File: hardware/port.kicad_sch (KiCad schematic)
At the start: 13 parts, among them J1 USB_A_Stacked, Q1 AO3401A, Q2 AO3401A, Q3 MMBT3904, Q4 MMBT3904

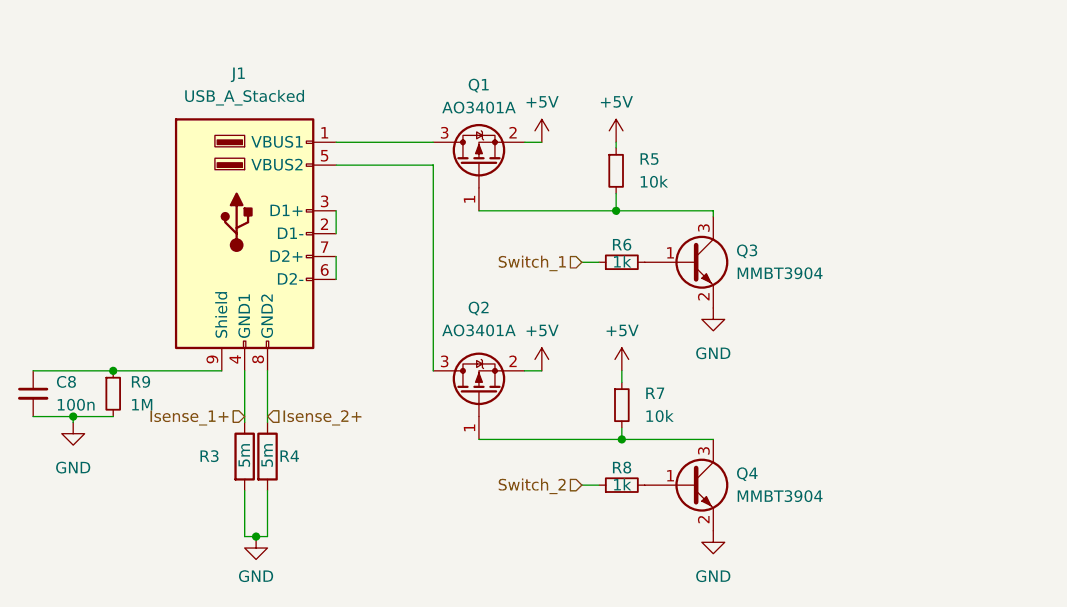
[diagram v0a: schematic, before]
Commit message: rev2
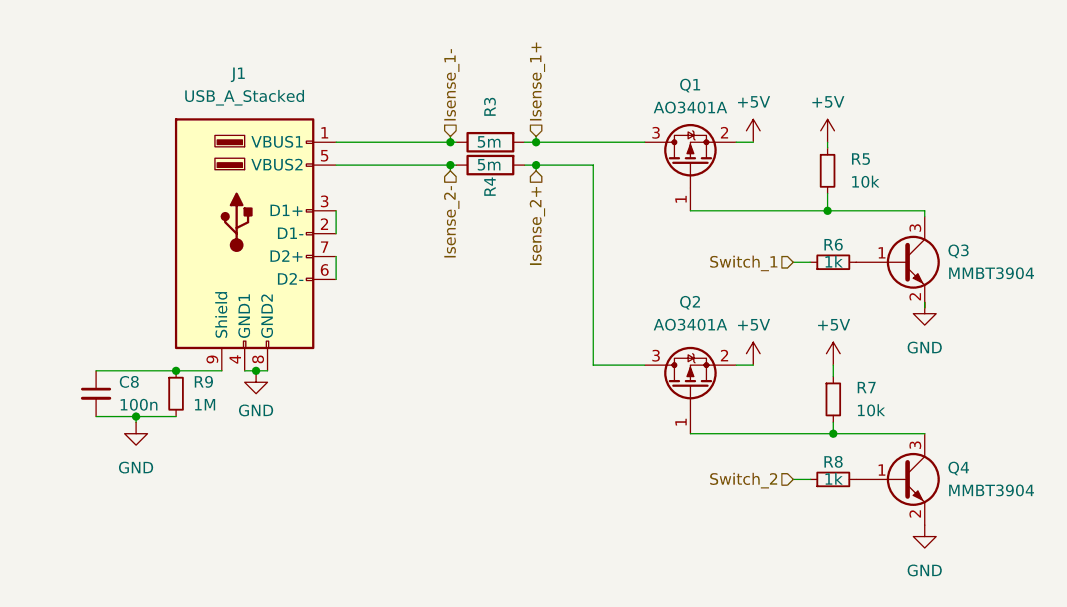
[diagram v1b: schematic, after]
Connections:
- net GND: now also J1.4 (GND1), J1.8 (GND2); no longer R3.2, R4.2
- net Isense_1+: now also Q1.3 (D), R3.2; no longer J1.4 (GND1), R3.1
- net Isense_2+: now also Q2.3 (D), R4.2; no longer J1.8 (GND2), R4.1
- net Isense_1-: now reaches J1.1 (VBUS1)
- net Isense_1-: now also R3.1; no longer Q1.3 (D)
- net Isense_2-: now reaches J1.5 (VBUS2)
- net Isense_2-: now also R4.1; no longer Q2.3 (D)
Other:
- moved on the sheet: C8, Q1, Q2, Q3, Q4, R5, R6, R7, R8, R9
